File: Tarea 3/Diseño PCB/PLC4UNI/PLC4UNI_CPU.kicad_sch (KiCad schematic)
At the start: 6 parts, among them U1 ESP32-S3-WROOM-1

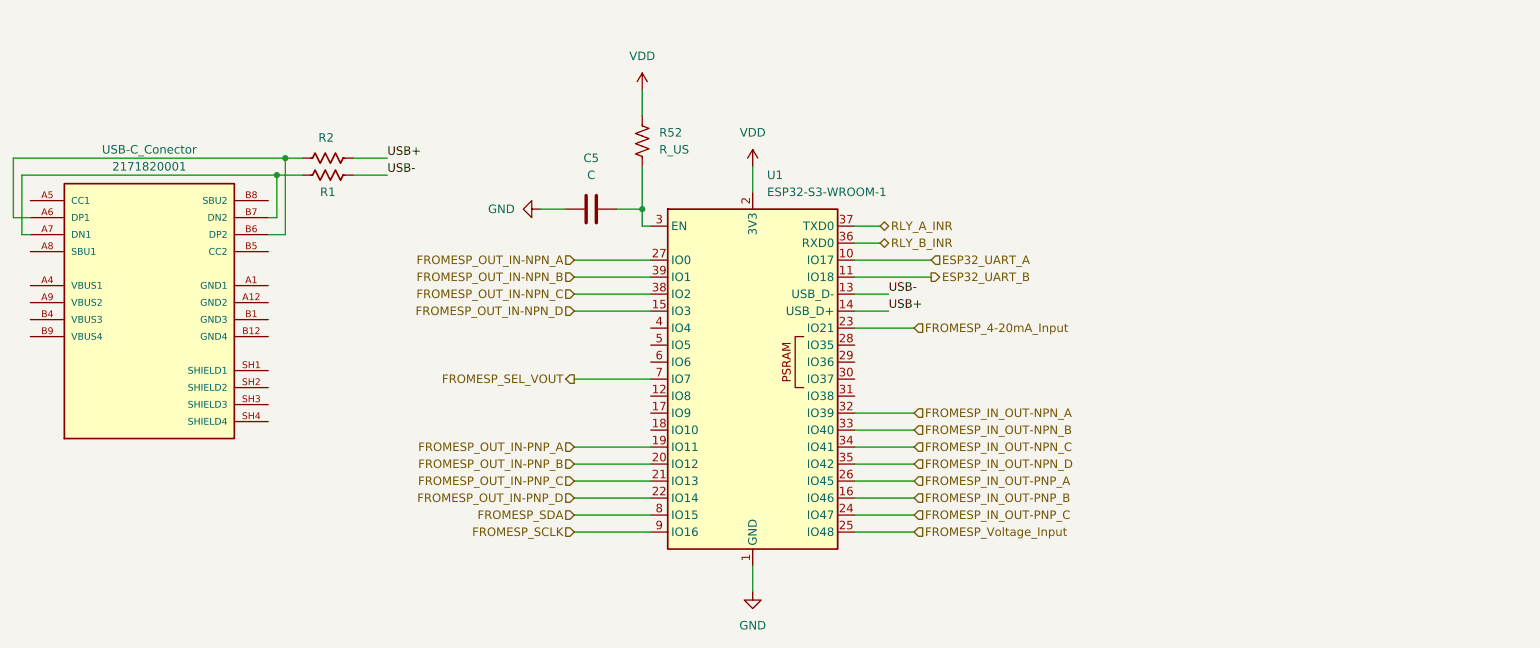
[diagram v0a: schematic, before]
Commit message: Tarea  3
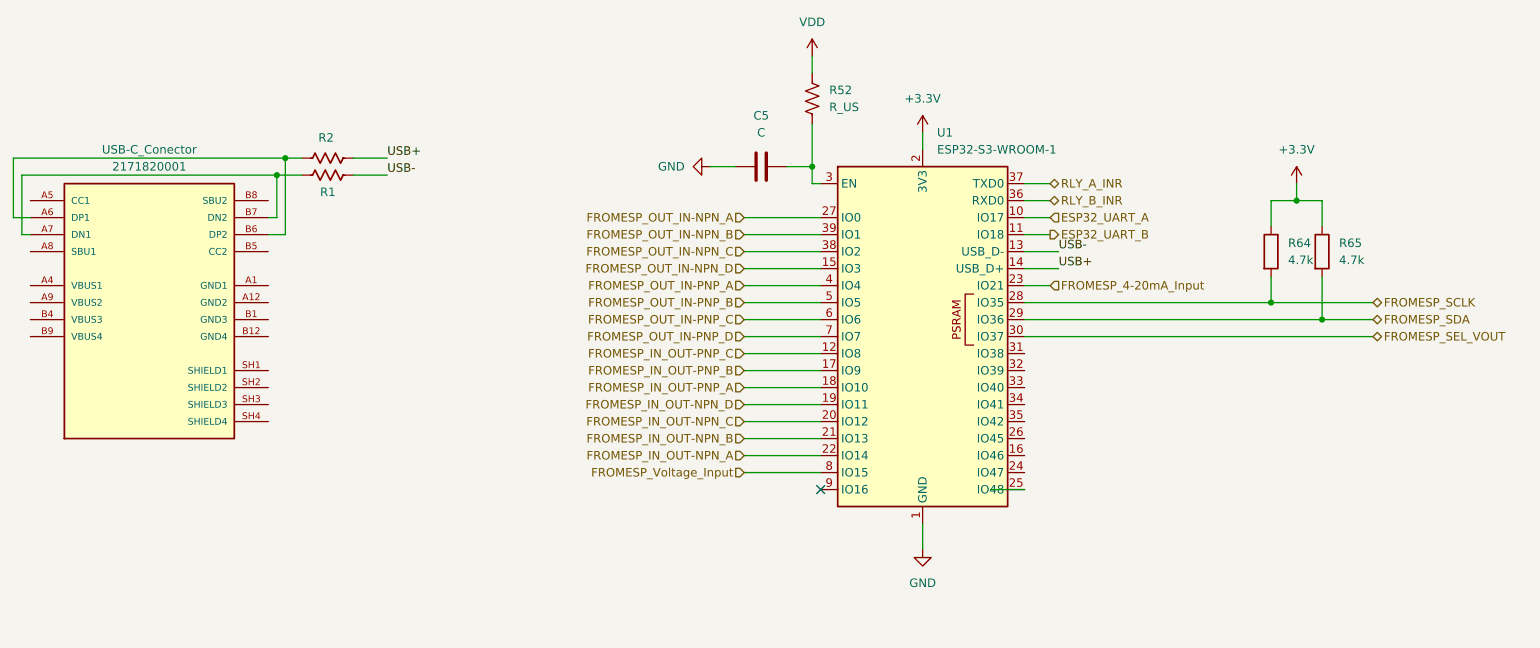
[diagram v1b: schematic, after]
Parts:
- added R64, R65: 4.7k, Resistor_SMD:R_0603_1608Metric, symbol Device:R
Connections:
- net FROMESP_IN_OUT-NPN_A: now also U1.22 (IO14); no longer U1.32 (IO39)
- net FROMESP_IN_OUT-NPN_B: now also U1.21 (IO13); no longer U1.33 (IO40)
- net FROMESP_IN_OUT-NPN_C: now also U1.20 (IO12); no longer U1.34 (IO41)
- net FROMESP_IN_OUT-NPN_D: now also U1.19 (IO11); no longer U1.35 (IO42)
- net FROMESP_IN_OUT-PNP_A: now also U1.18 (IO10); no longer U1.26 (IO45)
- net FROMESP_IN_OUT-PNP_B: now also U1.17 (IO9); no longer U1.16 (IO46)
- net FROMESP_IN_OUT-PNP_C: now also U1.12 (IO8); no longer U1.24 (IO47)
- net FROMESP_OUT_IN-PNP_A: now also U1.4 (IO4); no longer U1.19 (IO11)
- net FROMESP_OUT_IN-PNP_B: now also U1.5 (IO5); no longer U1.20 (IO12)
- net FROMESP_OUT_IN-PNP_C: now also U1.6 (IO6); no longer U1.21 (IO13)
- net FROMESP_OUT_IN-PNP_D: now also U1.7 (IO7); no longer U1.22 (IO14)
- net FROMESP_SCLK: now also U1.28 (IO35), R64.2; no longer U1.9 (IO16)
- net FROMESP_SDA: now also U1.29 (IO36), R65.2; no longer U1.8 (IO15)
- net FROMESP_SEL_VOUT: now also U1.30 (IO37); no longer U1.7 (IO7)
- net FROMESP_Voltage_Input: now also U1.8 (IO15); no longer U1.25 (IO48)
- net VDD: no longer U1.2 (3V3)
- new net +3.3V: R64.1, R65.1, U1.2 (3V3)
- no-connect marks 0 -> 1
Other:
- moved on the sheet: C5, R52, U1
